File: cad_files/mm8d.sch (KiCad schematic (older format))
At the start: 77 parts, among them J1 Screw_Terminal_1x05, J10 Screw_Terminal_1x05, J2 Screw_Terminal_1x04, J3 Screw_Terminal_1x04, J4 Screw_Terminal_1x04, J5 Screw_Terminal_1x04, J6 Screw_Terminal_1x03, J7 Screw_Terminal_1x03, J8 Screw_Terminal_1x03, J9 Screw_Terminal_1x03, K1 LEG-5, K2 LEG-5, K3 LEG-5, K4 LEG-5, Q1 BC548C, Q2 BC548C, Q3 BC548C, Q4 BC548C, Q5 BC548C, Q6 BC548C, Q7 BC548C, Q8 BC548C, U1 4N25, U2 4N25, U3 4N25, U4 4N25, U5 74LS14, U6 74LS05

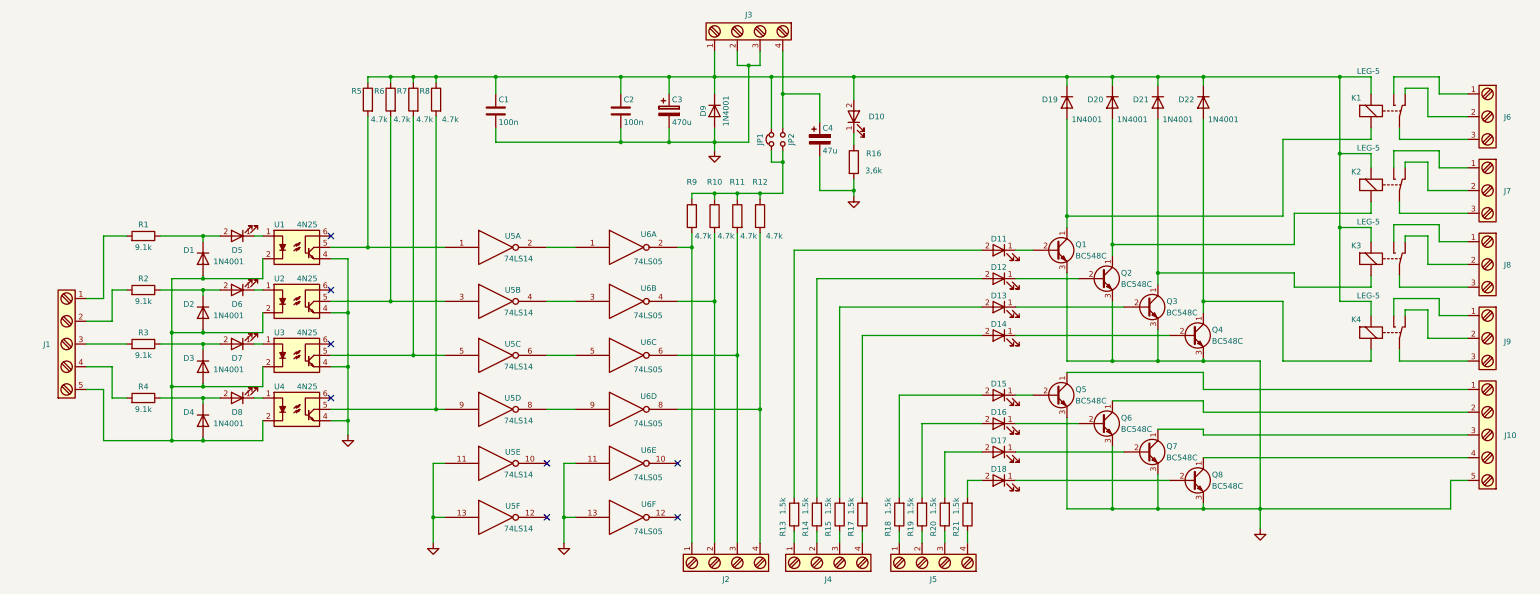
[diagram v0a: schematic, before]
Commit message: 210325
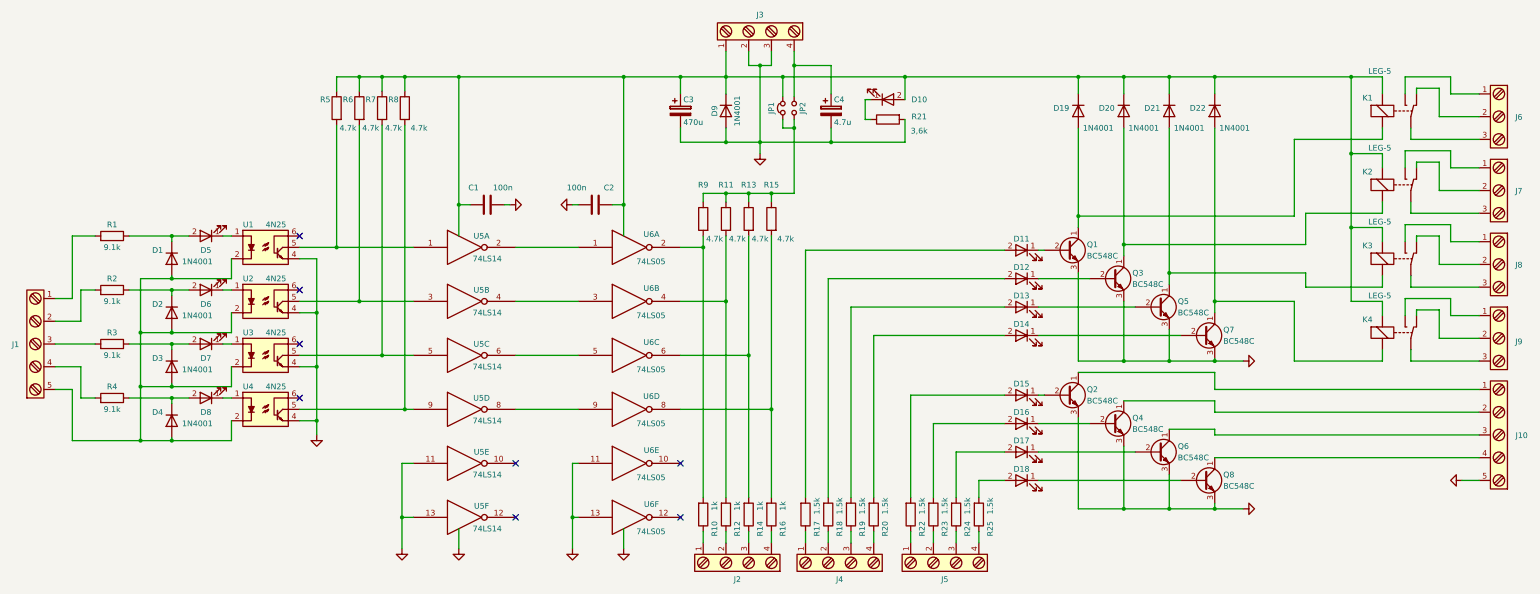
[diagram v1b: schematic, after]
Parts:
- added R10, R12, R14, R16: 1k, Discret:R5, symbol R
- C4: value 47u -> 4.7u; footprint Capacitors_THT:C_Radial_D8_L11.5_P3.5 -> Capacitors_THT:C_Radial_D5_L11_P2.5
- K1, K2, K3, K4: footprint (none) -> Discret:relay_leg
- R1, R2, R3, R4, R5, R6, R7, R8, R9: footprint Discret:R4 -> Discret:R5
- R11: renamed from R10; footprint Discret:R4 -> Discret:R5
- R13: renamed from R11; footprint Discret:R4 -> Discret:R5
- R15: renamed from R12; footprint Discret:R4 -> Discret:R5
- R17: renamed from R13; footprint Discret:R4 -> Discret:R5
- R18: renamed from R14; footprint Discret:R4 -> Discret:R5
- R19: renamed from R15; footprint Discret:R4 -> Discret:R5
- R20: renamed from R17; footprint Discret:R4 -> Discret:R5
- R21: renamed from R16; footprint Discret:R4 -> Discret:R5
- R22: renamed from R18; footprint Discret:R4 -> Discret:R5
- R23: renamed from R19; footprint Discret:R4 -> Discret:R5
- R24: renamed from R20; footprint Discret:R4 -> Discret:R5
- R25: renamed from R21; footprint Discret:R4 -> Discret:R5
- renumbered C2 to C1, C1 to C2, Q5 to Q2, Q2 to Q3, Q6 to Q4, Q3 to Q5, Q7 to Q6, Q4 to Q7
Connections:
- net GNDD is gone; now on net GND: C1.2, C2.2, C3.2, C4.2, D9.2 (A), J10.5, J3.2, J3.3, Q1.3 (E), Q2.3 (E), Q3.3 (E), Q4.3 (E), Q5.3 (E), Q6.3 (E), Q7.3 (E), Q8.3 (E), R21.2, U1.4, U2.4, U3.4, U4.4, U5.11, U5.13, U6.11, U6.13
- net VCC: now also C1.1, C2.1, C3.1, D10.2 (A), D19.1 (K), D20.1 (K), D21.1 (K), D22.1 (K), D9.1 (K), J3.1, JP1.2, K1.1 (Coil), K2.1 (Coil), K3.1 (Coil), K4.1 (Coil), R5.1, R6.1, R7.1, R8.1
- net at R9.2, U6.2: now also R10.2; no longer J2.1
- net at R11.2, U6.4: now also R12.2; no longer J2.2
- net at R13.2, U6.6: now also R14.2; no longer J2.3
- net at R15.2, U6.8: now also R16.2; no longer J2.4
- new net: J2.1, R10.1
- new net: J2.2, R12.1
- new net: J2.3, R14.1
- new net: J2.4, R16.1
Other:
- moved on the sheet: C1, C2, C3, C4, D1, D10, D11, D12, D13, D14, D15, D16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

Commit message: 210325
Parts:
- C1, C2: footprint Capacitors_THT:C_Rect_L7_W2.5_P5 -> Capacitors_THT:C_Rect_L7.0mm_W2.5mm_P5.00mm
- C3: footprint Capacitors_THT:C_Radial_D8_L11.5_P3.5 -> Capacitors_THT:CP_Radial_D8.0mm_P3.50mm
- C4: footprint Capacitors_THT:C_Radial_D5_L11_P2.5 -> Capacitors_THT:CP_Radial_D5.0mm_P2.50mm
- D1, D19, D2, D20, D21, D22, D3, D4, D9: footprint Diodes_THT:Diode_DO-41_SOD81_Horizontal_RM10 -> Diodes_THT:D_DO-41_SOD81_P10.16mm_Horizontal
- D10, D11, D12, D13, D14, D15, D16, D17, D18, D5, D6, D7, D8: footprint LEDs:LED-3MM -> LEDs:LED_D3.0mm
- JP1, JP2: footprint Socket_Strips:Socket_Strip_Straight_1x02 -> Socket_Strips:Socket_Strip_Straight_1x02_Pitch2.54mm
- K1, K2, K3, K4: footprint Discret:relay_leg -> relay_lg:relay_leg
- R1, R10, R11, R12, R13, R14, R15, R16, R17, R18, R19, R2, R20, R21, R22, R23, R24, R25, R3, R4, R5, R6, R7, R8, R9: footprint Discret:R5 -> Resistors_THT:R_Axial_DIN0411_L9.9mm_D3.6mm_P12.70mm_Horizontal
